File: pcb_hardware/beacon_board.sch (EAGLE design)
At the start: 66 parts, among them IC1-AVR ATMEGA32U4TQFP, J1-ISP AVR_SPI_PRG_6PTH, Q1 PZT2222A, Q2 PZT2222A, Q3 PZT2222A, Q4 PZT2222A, Q5 PZT2222A, Q6 PZT2222A, Q7 PZT2222A, Y1 16MHz

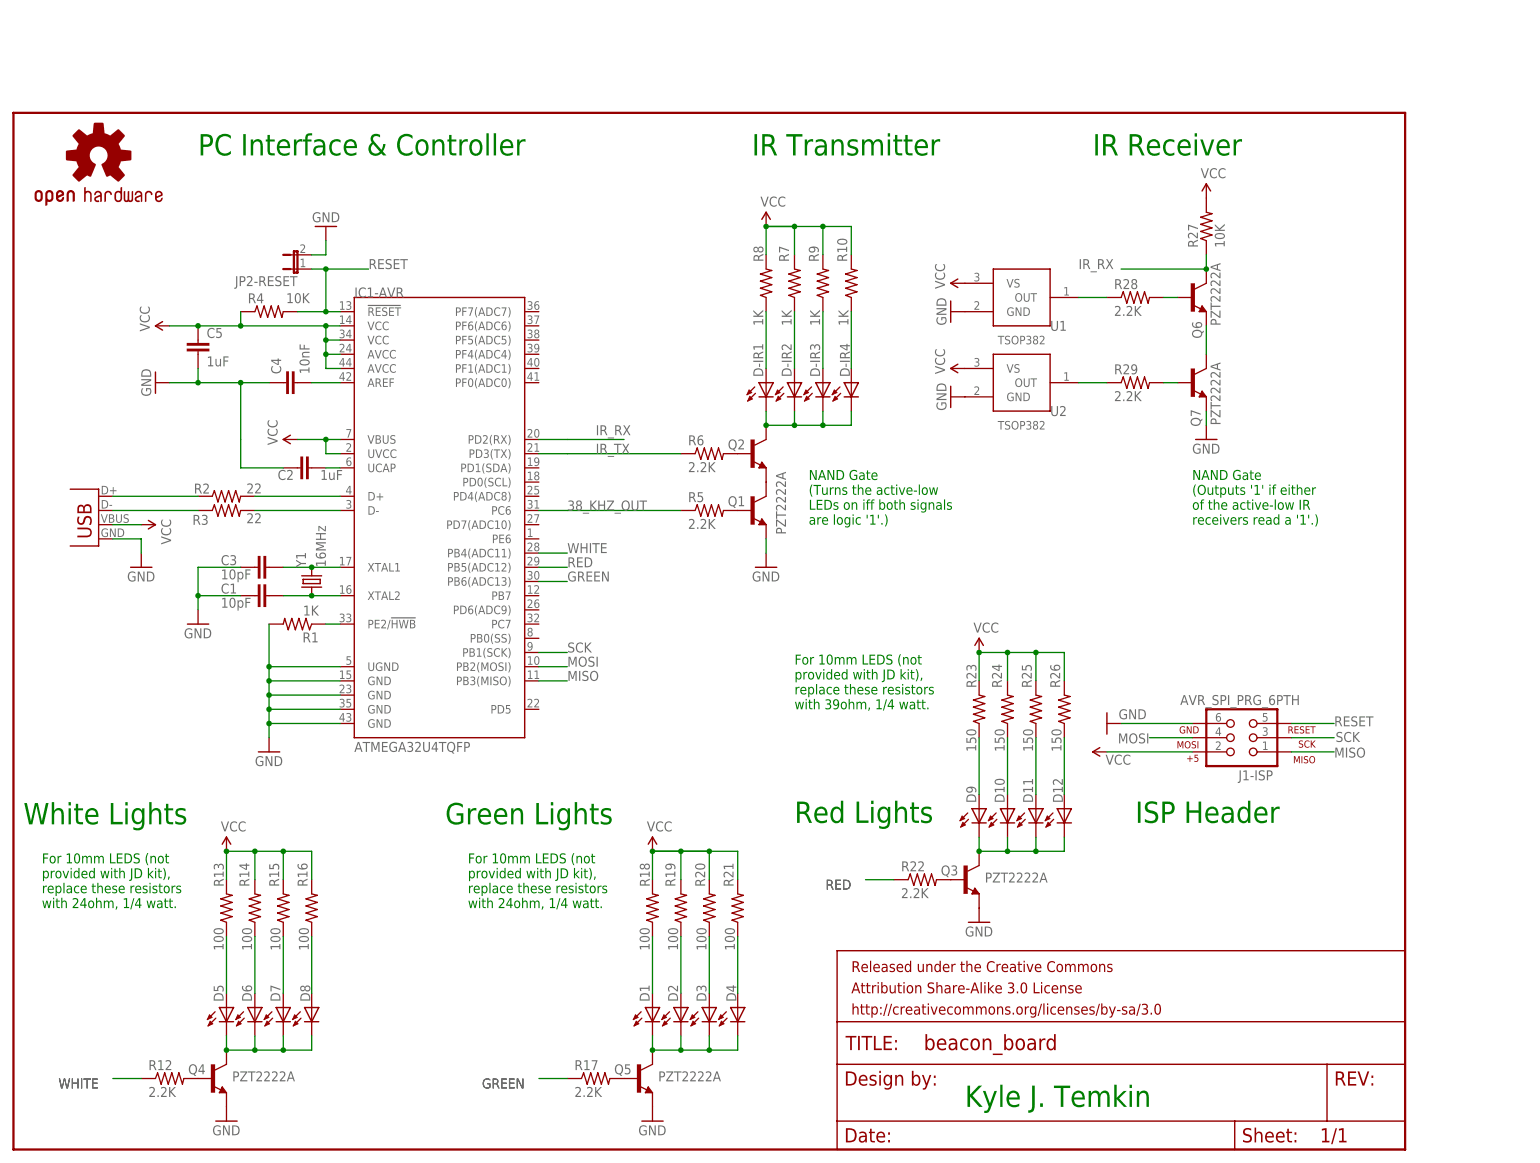
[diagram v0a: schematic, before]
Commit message: Complete alpha prototype for PCB
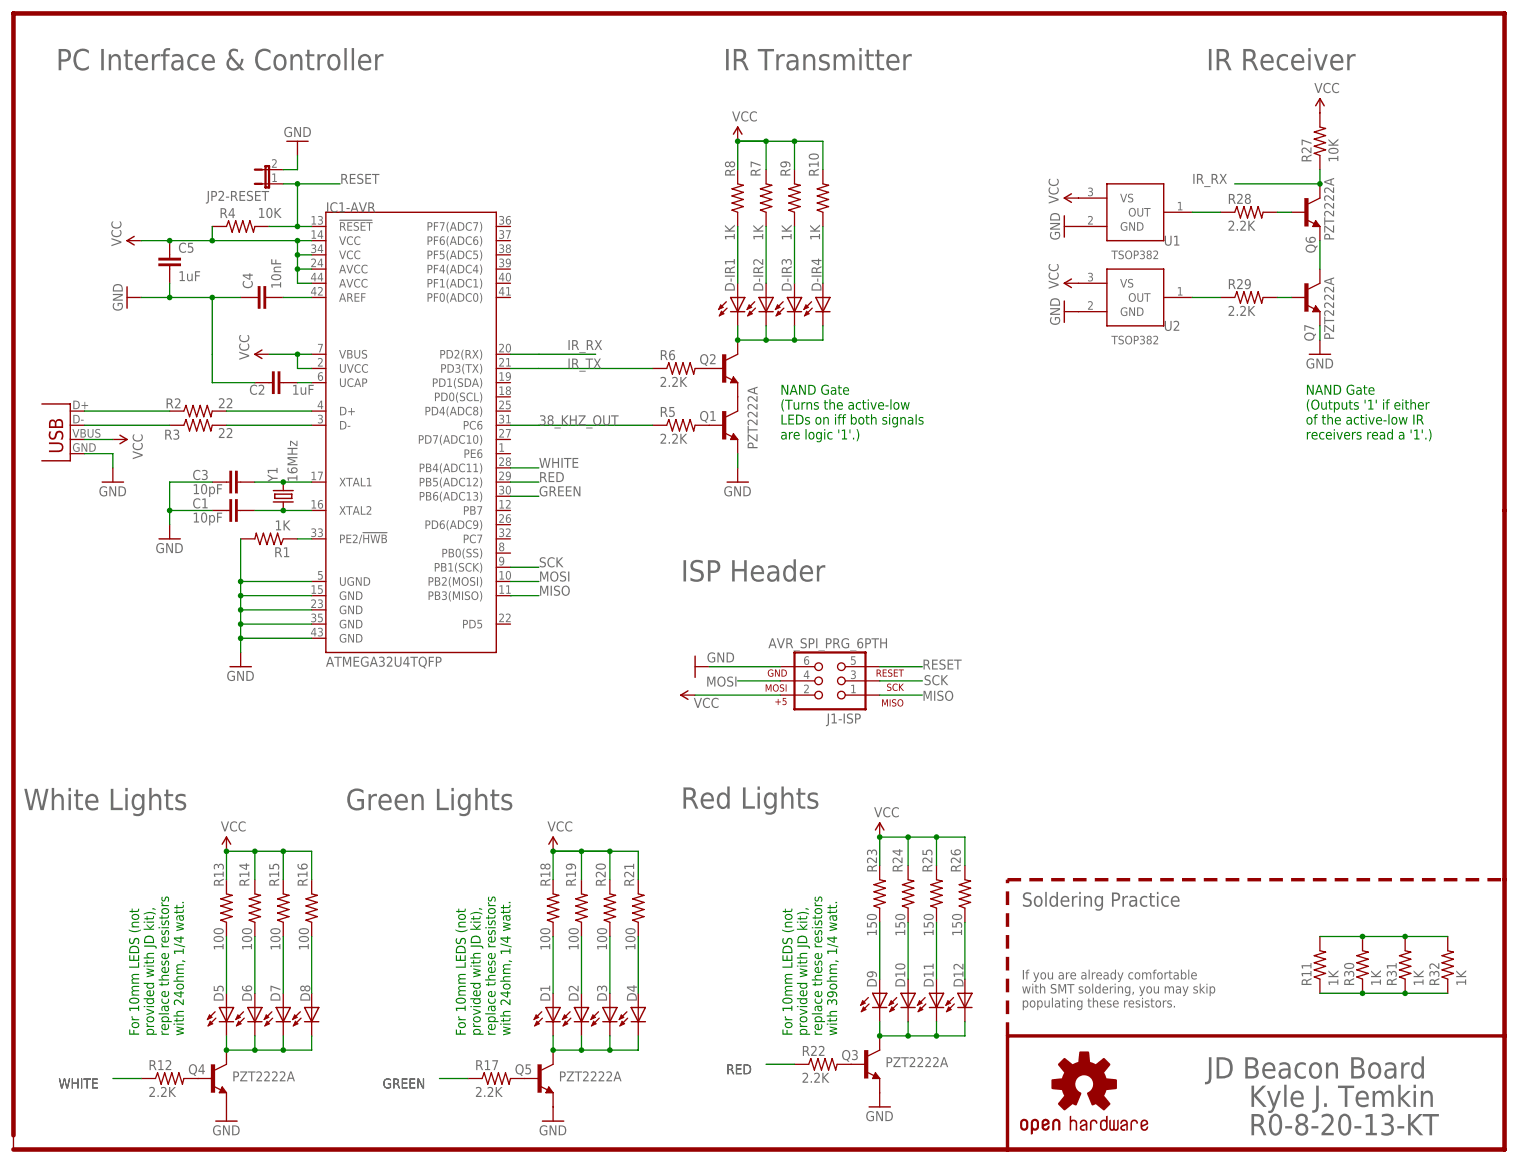
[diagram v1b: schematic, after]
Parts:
- removed FRAME1: FRAME-LETTER, SparkFun-Aesthetics:FRAME-LETTER
- added R11, R30, R31, R32: 1K, SparkFun-Passives:RESISTOR0805-RES
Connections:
- new net N$30: R11.2, R30.2, R31.2, R32.2
- new net N$31: R11.1, R30.1, R31.1, R32.1
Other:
- note added: "If you are already comfortable with SMT soldering, you may skip populating these resistors."
- note added: "JD Beacon Board"
- note added: "R0-8-20-13-KT"
- note added: "Soldering Practice"
- moved on the sheet: C1, C2, C3, C4, C5, D-IR1, D-IR2, D-IR3, D-IR4, D1, D10, D11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
